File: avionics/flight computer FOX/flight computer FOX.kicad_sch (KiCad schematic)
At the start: 25 parts, among them J1 Screw_Terminal_01x02, J2 Conn_01x03, J3 Conn_01x03, J4 Conn_01x03, J5 Conn_01x03, J6 Conn_01x03, J7 Screw_Terminal_01x02, J8 Screw_Terminal_01x02, Q1 IRF540N, Q2 IRF540N, U1 ESP32-DevKitC, U2 LM7805_TO220

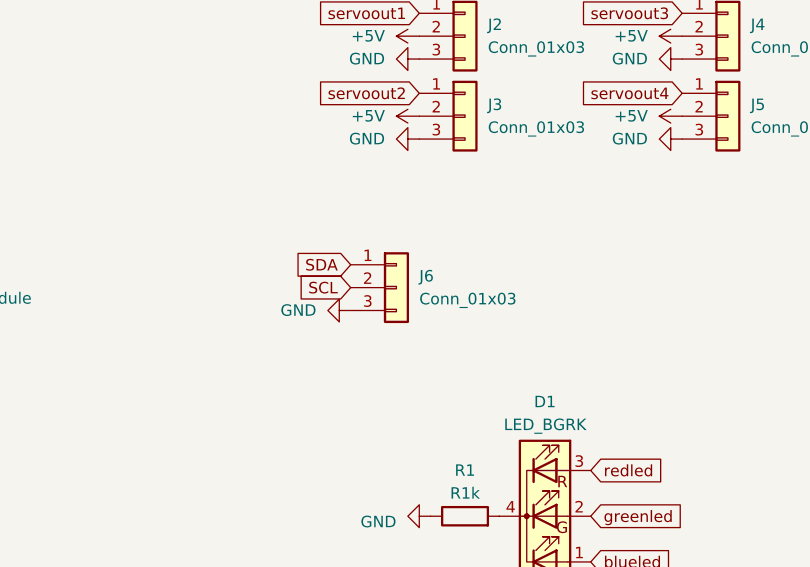
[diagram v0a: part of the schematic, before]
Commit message: stuff
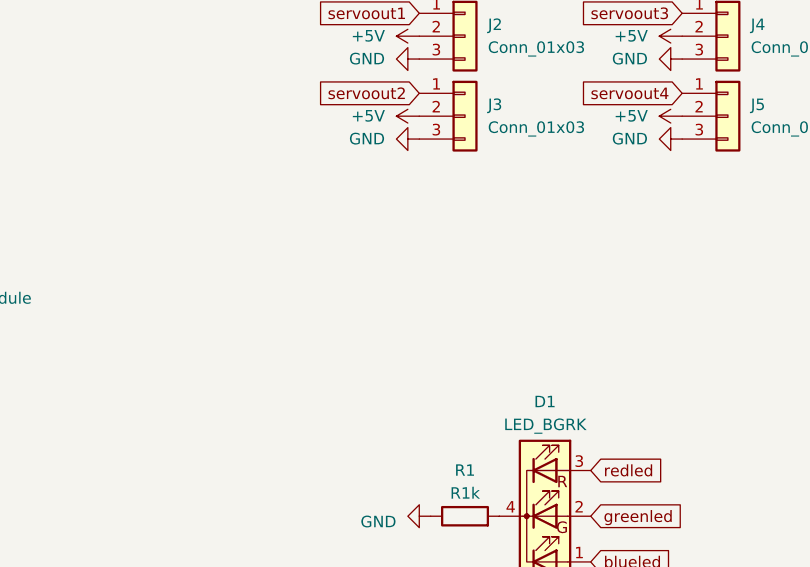
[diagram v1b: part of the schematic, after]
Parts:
- removed J6: Conn_01x03, Connector_PinHeader_2.54mm:PinHeader_1x03_P2.54mm_Vertical, symbol Connector_Generic:Conn_01x03
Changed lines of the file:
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@@
-    )
-  )
-  (global_label "SDA" (shape input) (at 123.19 53.34 180) (fields_autoplaced)
-    (effects (font (size 1.27 1.27)) (justify right))
-    (property "Intersheetrefs" "${INTERSHEET_REFS}" (at 116.7161 53.34 0)
-      (effects (font (size 1.27 1.27)) (justify right) hide)
-    )
-  )
-  (global_label "SCL" (shape input) (at 123.19 55.88 180) (fields_autoplaced)
-    (effects (font (size 1.27 1.27)) (justify right))
-    (property "Intersheetrefs" "${INTERSHEET_REFS}" (at 116.7766 55.88 0)
-      (effects (font (size 1.27 1.27)) (justify right) hide)
     )
   )
@@
     )
   )
-  (symbol (lib_id "power:GND") (at 123.19 58.42 270) (unit 1)
-    (in_bom yes) (on_board yes) (dnp no) (fields_autoplaced)
-    (property "Reference" "#PWR033" (at 116.84 58.42 0)
-      (effects (font (size 1.27 1.27)) hide)
-    )
-    (property "Value" "GND" (at 119.38 58.42 90)
-      (effects (font (size 1.27 1.27)) (justify right))
-    )
-    (property "Footprint" "" (at 123.19 58.42 0)
-      (effects (font (size 1.27 1.27)) hide)
-    )
-    (property "Datasheet" "" (at 123.19 58.42 0)
-      (effects (font (size 1.27 1.27)) hide)
-    )
-    (pin "1")
-    (instances
-      (project "flight computer FOX"
-        (path "/05785e23-8de8-49cd-8fd9-ec33b4a12221"
-          (reference "#PWR033") (unit 1)
-        )
-      )
-    )
-  )
   (symbol (lib_id "Transistor_FET:IRF540N") (at 241.3 139.7 0) (unit 1)
     (in_bom yes) (on_board yes) (dnp no) (fields_autoplaced)
@@
         )
       )
-    )
-  )
-  (symbol (lib_id "Connector_Generic:Conn_01x03") (at 128.27 55.88 0) (unit 1)
-    (in_bom yes) (on_board yes) (dnp no) (fields_autoplaced)
-    (property "Reference" "J6" (at 130.81 54.61 0)
-      (effects (font (size 1.27 1.27)) (justify left))
-    )
-    (property "Value" "Conn_01x03" (at 130.81 57.15 0)
-      (effects (font (size 1.27 1.27)) (justify left))
-    )
-    (property "Footprint" "Connector_PinHeader_2.54mm:PinHeader_1x03_P2.54mm_Vertical" (at 128.27 55.88 0)
-      (effects (font (size 1.27 1.27)) hide)
-    )
-    (property "Datasheet" "~" (at 128.27 55.88 0)
-      (effects (font (size 1.27 1.27)) hide)
-    )
-    (pin "1")
-    (pin "2")
-    (pin "3")
-    (instances
-      (project "flight computer FOX"
-        (path "/05785e23-8de8-49cd-8fd9-ec33b4a12221"
-          (reference "J6") (unit 1)
-        )
-      )
